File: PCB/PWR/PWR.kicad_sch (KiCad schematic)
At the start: 1 part

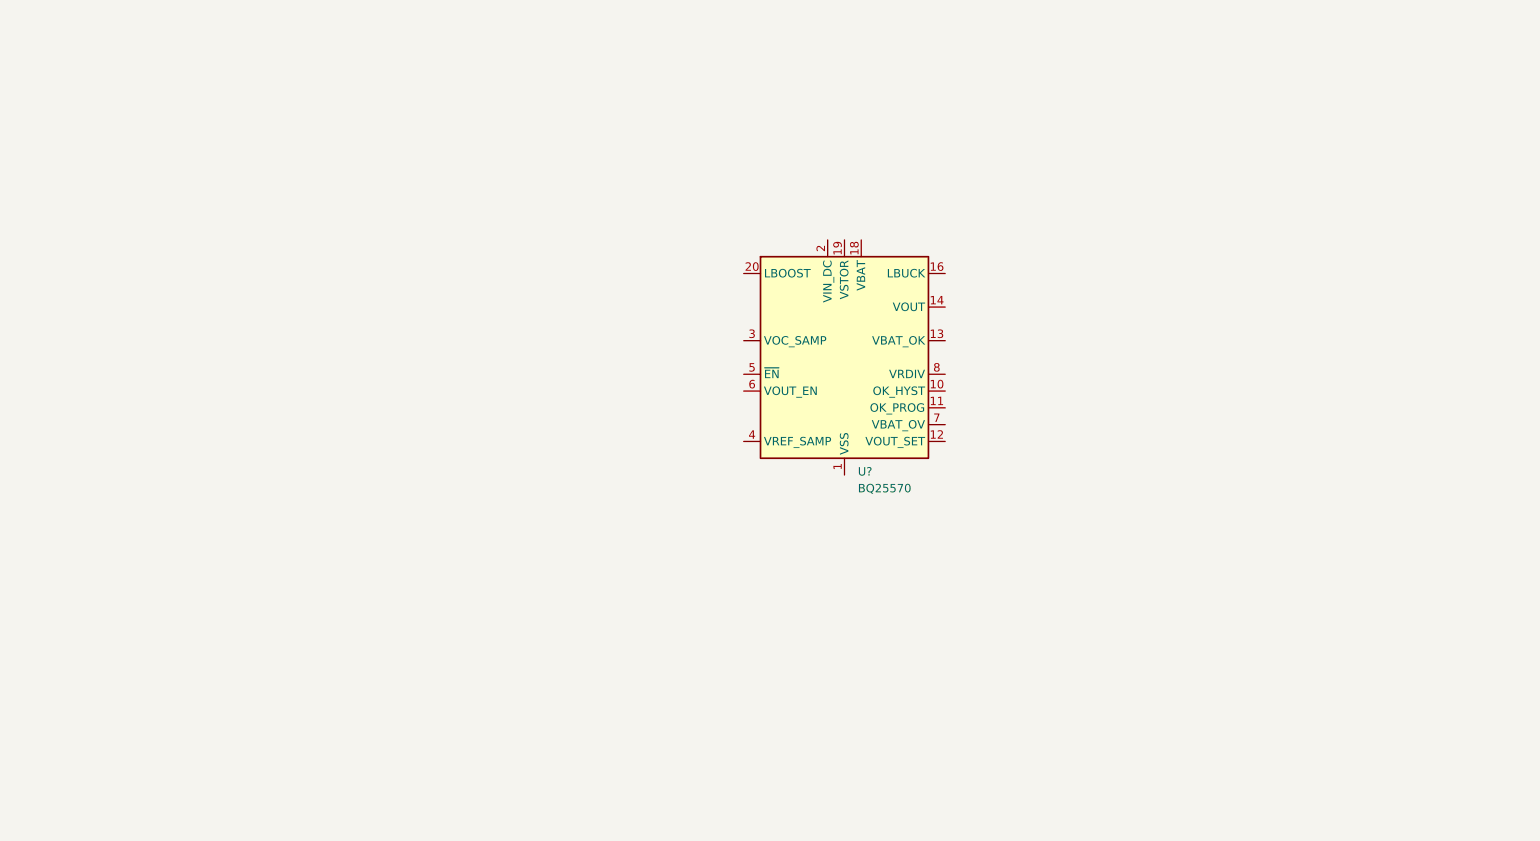
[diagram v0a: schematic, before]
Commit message: udated by FZ from Windows
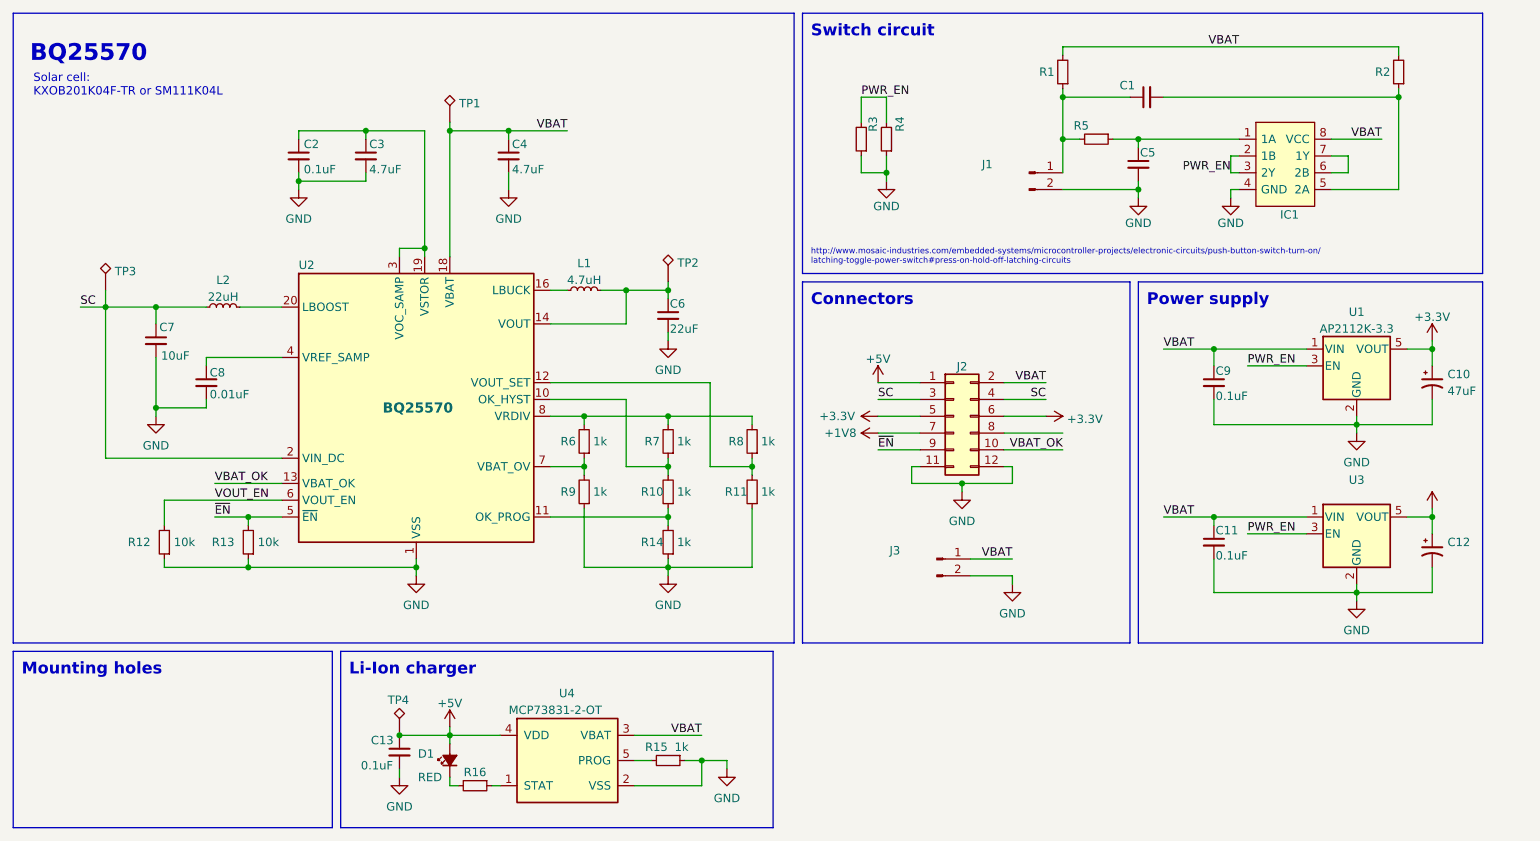
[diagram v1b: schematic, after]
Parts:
- added C1, C5: (no value), symbol Device:C_Small
- added C10: 47uF, symbol Device:C_Polarized_Small_US
- added C11, C13, C2, C9: 0.1uF, symbol Device:C_Small
- added C12: (no value), symbol Device:C_Polarized_Small_US
- added C3, C4: 4.7uF, symbol Device:C_Small
- added C6: 22uF, symbol Device:C_Small
- added C7: 10uF, symbol Device:C_Small
- added C8: 0.01uF, symbol Device:C_Small
- added D1: RED, symbol Device:LED_Small_Filled
- added IC1: (no value), symbol SamacSys_Parts:SN74LVC2G00DCURE4
- added J1, J3: (no value), symbol Connector:Conn_01x02_Male
- added J2: (no value), symbol Connector_Generic:Conn_02x06_Odd_Even
- added L1: 4.7uH, symbol Device:L_Small
- added L2: 22uH, symbol Device:L_Small
- added R1, R16, R2, R3, R4, R5: (no value), symbol Device:R_Small
- added R10, R11, R14, R15, R6, R7, R8, R9: 1k, symbol Device:R_Small
- added R12, R13: 10k, symbol Device:R_Small
- added TP1, TP2, TP3, TP4: TestPoint_Alt, symbol Connector:TestPoint_Alt
- added U1: AP2112K-3.3, Package_TO_SOT_SMD:SOT-23-5, symbol Regulator_Linear:AP2112K-3.3
- added U3: (no value), symbol Regulator_Linear:AP2112K-1.8
- added U4: MCP73831-2-OT, Package_TO_SOT_SMD:SOT-23-5, symbol Battery_Management:MCP73831-2-OT
- gave numbers to parts that had none: 1
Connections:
- net GND: now reaches U2.1 (VSS), U2.15 (VSS), U2.17 (VSS), U2.21 (VSS), U2.9 (VSS)
- net GND: now also C10.2, C11.2, C12.2, C13.2, C2.2, C3.2, C4.2, C5.2, C6.2, C7.2, C8.2, C9.2, IC1.4 (GND), J1.2 (Pin_2), J2.11 (Pin_11), J2.12 (Pin_12), J3.2 (Pin_2), R11.1, R12.1, R13.1, R14.1, R15.1, R3.1, R4.1, R9.1, U1.2 (GND), U3.2 (GND), U4.2 (VSS)
- net at U2.10 (OK_HYST): now also R10.2, R7.1
- net at U2.11 (OK_PROG): now also R10.1, R14.2
- net at U2.12 (VOUT_SET): now also R11.2, R8.1
- net VBAT_OK: now reaches U2.13 (VBAT_OK)
- net VBAT_OK: now also J2.10 (Pin_10)
- net at U2.14 (VOUT): now also C6.1, L1.2, TP2.1
- net at U2.16 (LBUCK): now also L1.1
- net VBAT: now reaches U2.18 (VBAT)
- net VBAT: now also C11.1, C4.1, C9.1, IC1.8 (VCC), J2.2 (Pin_2), J3.1 (Pin_1), R1.2, R2.2, TP1.1, U1.1 (VIN), U3.1 (VIN), U4.3 (VBAT)
- net at U2.19 (VSTOR): now also U2.3 (VOC_SAMP), C2.1, C3.1
- net SC: now reaches U2.2 (VIN_DC)
- net SC: now also C7.1, J2.3 (Pin_3), J2.4 (Pin_4), L2.1, TP3.1
- net at U2.20 (LBOOST): now also L2.2
- net at U2.4 (VREF_SAMP): now also C8.1
- net ~{EN}: now reaches U2.5 (~{EN})
- net ~{EN}: now also J2.9 (Pin_9), R13.2
- net VOUT_EN: now reaches U2.6 (VOUT_EN)
- net VOUT_EN: now also R12.2
- net at U2.7 (VBAT_OV): now also R6.1, R9.2
- net at U2.8 (VRDIV): now also R6.2, R7.2, R8.2
- new net: C1.2, IC1.5 (2A), R2.1
- new net: C5.1, IC1.1 (1A), R5.1
- new net: C1.1, J1.1 (Pin_1), R1.1, R5.2
- new net: IC1.6 (2B), IC1.7 (1Y)
- new net: R16.1, U4.1 (STAT)
- new net: D1.1 (K), R16.2
- new net: R15.2, U4.5 (PROG)
- new net +1V8: C12.1, J2.7 (Pin_7), U3.5 (VOUT)
- new net +3V3: C10.1, J2.5 (Pin_5), J2.6 (Pin_6), U1.5 (VOUT)
- new net +5V: C13.1, D1.2 (A), J2.1 (Pin_1), TP4.1, U4.4 (VDD)
- new net PWR_EN: IC1.2 (1B), IC1.3 (2Y), R3.2, R4.2, U1.3 (EN), U3.3 (EN)
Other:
- note added: "BQ25570"
- note added: "Connectors"
- note added: "Li-Ion charger"
- note added: "Mounting holes"
- note added: "Power supply"
- note added: "Solar cell: KXOB201K04F-TR or SM111K04L"
- note added: "Switch circuit"
- note added: "http://www.mosaic-industries.com/embedded-systems/microcontroller-projects/electronic-circuits/push-button-switch-turn-on/ latching-toggle-power-switch#press-on-hold-off-latching-circuits"
- company: (none) -> MIT Media Lab
- title: (none) -> HexSense Svalbard - PWR
- moved on the sheet: U2
